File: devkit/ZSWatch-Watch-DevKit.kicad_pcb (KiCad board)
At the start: 4 copper layers, 100 x 70 mm, 129 parts, among them IC401 nPM1300-QEXX, IC501 APDS-9306-065, IC502 BMI270, IC503 LIS2MDLTR, IC504 BMP581, IC505 DRV2603RUNT, IC506 PCA9306JK, IC507 RV-8263-C8, IC601 FAN5622SX, IC602 USBLC6-2P6, IC603 MX25U51245GZ4I00, IC604 NTS0104GU12, M601 NORA-B106, Q401 PMZ550UNEYL, Q402 PMZ550UNEYL, Q403 PMZ550UNEYL, Q404 PMZB320UPEYL, X401 Battery, X402 Battery, X403 Power, X501 Current, X502 I2S, X503 Current, X504 I2C, X505 Current, X506 Current, X507 Current, X508 Current, X509 Motor, X510 Current, X601 DEBUG, X602 Current, X603 Device, X604 UART, X605 GPIO, X606 Current, X607 IO Current, X608 Display, X609 Touch Current, X610 LED Current

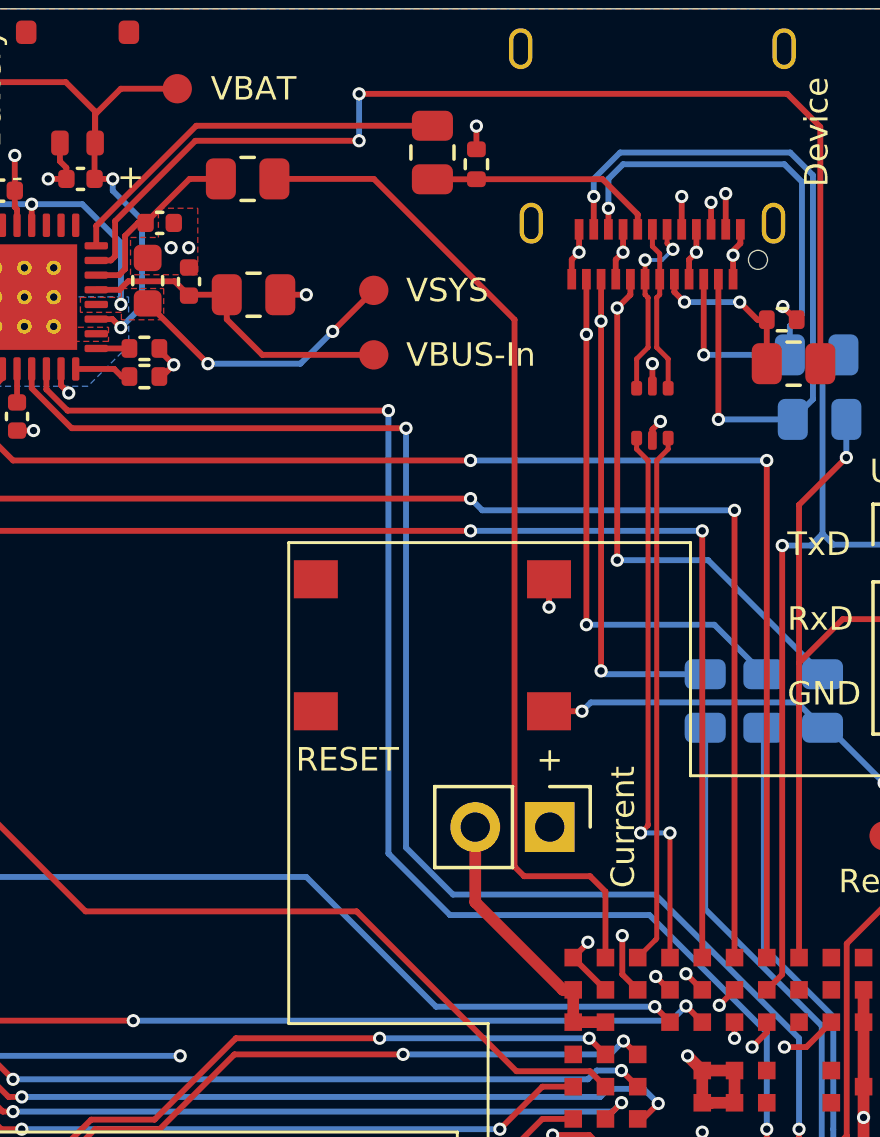
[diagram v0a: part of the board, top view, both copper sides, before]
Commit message: Revert "Feature: Issue #174"
This reverts commit a258055a47c56b8763088da3e06577d57b5d3abc.
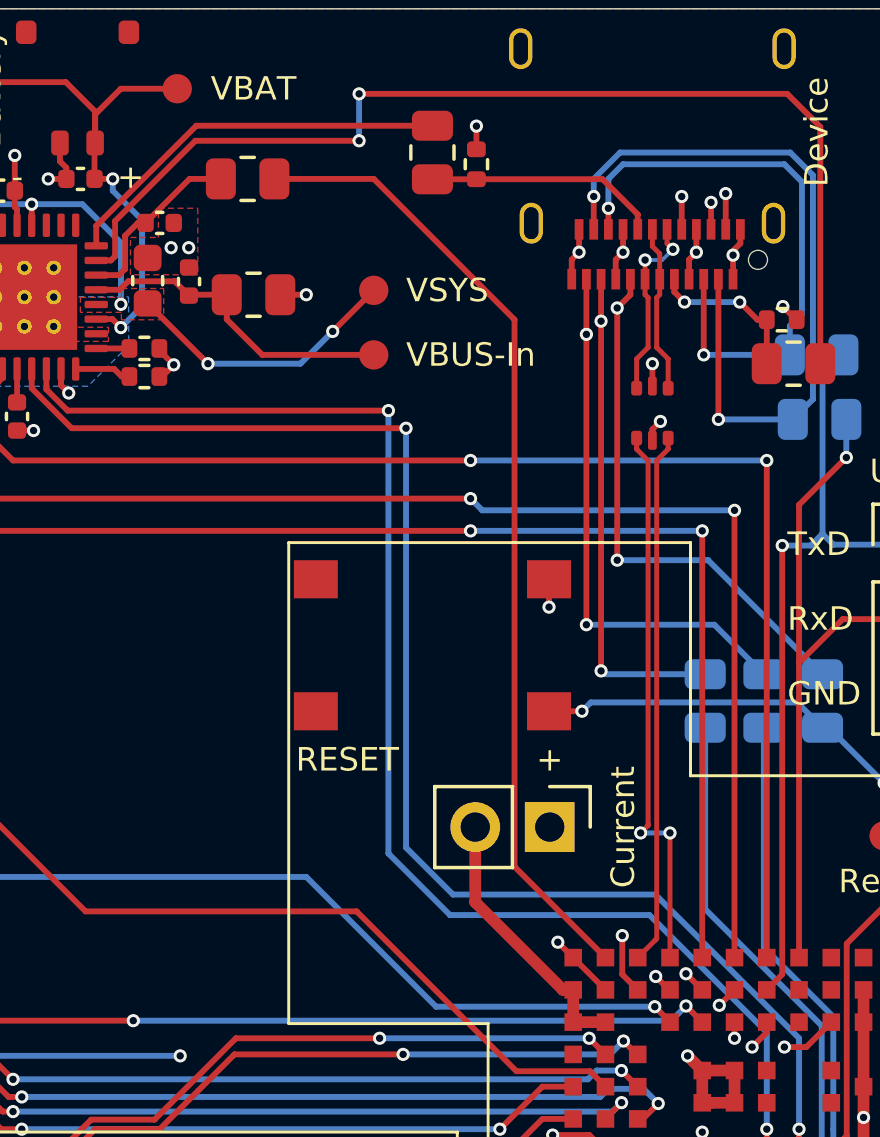
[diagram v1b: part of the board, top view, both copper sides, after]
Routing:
- net /Project Architecture/MCU/USB-VBUS-Out: track 34.5 -> 33.2 mm
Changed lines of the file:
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@@
 		)
 	)
-	(gr_poly
-		(pts
-			(xy 243.2 145.02092) (xy 242.8 145.42092) (xy 243.2 145.42092)
-		)
-		(stroke
-			(width 0.1)
-			(type solid)
-		)
-		(fill yes)
-		(layers "F.Cu" "F.Mask")
-	)
-	(gr_poly
-		(pts
-			(xy 242.8 156.07092) (xy 243.2 156.47092) (xy 243.2 156.07092)
-		)
-		(stroke
-			(width 0.1)
-			(type solid)
-		)
-		(fill yes)
-		(layers "F.Cu" "F.Mask")
-	)
 	(gr_rect
 		(start 172.1 116.2)
@@
 	)
 	(segment
-		(start 244.6 145.85)
-		(end 244.1 146.35)
-		(width 0.2)
-		(layer "F.Cu")
-		(net 1)
-	)
-	(segment
 		(start 170.61 141.1)
 		(end 170.61 140.7)
@@
 	)
 	(segment
+		(start 243.575 145.825)
+		(end 244.1 146.35)
+		(width 0.2)
+		(layer "F.Cu")
+		(net 1)
+	)
+	(segment
 		(start 236.62 175.4)
 		(end 236.62 174.775)
@@
 	)
 	(segment
-		(start 244.6 145.825)
-		(end 244.6 145.85)
-		(width 0.2)
-		(layer "F.Cu")
-		(net 1)
-	)
-	(segment
 		(start 201.99 145.1375)
 		(end 201.4 145.1375)
@@
 	)
 	(via
-		(at 244.6 145.825)
+		(at 243.575 145.825)
 		(size 0.45)
 		(drill 0.25)
@@
 	)
 	(segment
-		(start 242.1 124.6)
-		(end 237.3 119.8)
-		(width 0.2)
-		(layer "F.Cu")
-		(net 52)
-	)
-	(segment
-		(start 242.1 143.25)
+		(start 237.3 119.8)
 		(end 242.1 124.6)
 		(width 0.2)
@@
 	)
 	(segment
-		(start 245.2 146.35)
-		(end 245.2 144.1)
-		(width 0.2)
-		(layer "F.Cu")
-		(net 52)
-	)
-	(segment
-		(start 244.675 143.575)
-		(end 242.425 143.575)
-		(width 0.2)
-		(layer "F.Cu")
-		(net 52)
-	)
-	(segment
-		(start 245.2 144.1)
-		(end 244.675 143.575)
+		(start 242.1 143.25)
+		(end 245.2 146.35)
 		(width 0.2)
 		(layer "F.Cu")
@@
 	)
 	(segment
-		(start 237.3 119.8)
-		(end 233.9125 119.8)
+		(start 242.1 124.6)
+		(end 242.1 143.25)
 		(width 0.2)
 		(layer "F.Cu")
@@
 	)
 	(segment
-		(start 242.425 143.575)
-		(end 242.1 143.25)
+		(start 233.9125 119.8)
+		(end 237.3 119.8)
 		(width 0.2)
 		(layer "F.Cu")
